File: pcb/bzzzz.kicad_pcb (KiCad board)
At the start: 2 copper layers, 18.3 x 46.2 mm, 29 parts, among them J1 OUT, J2 OUT, Q1 FDD8424H, Q2 FDD8424H

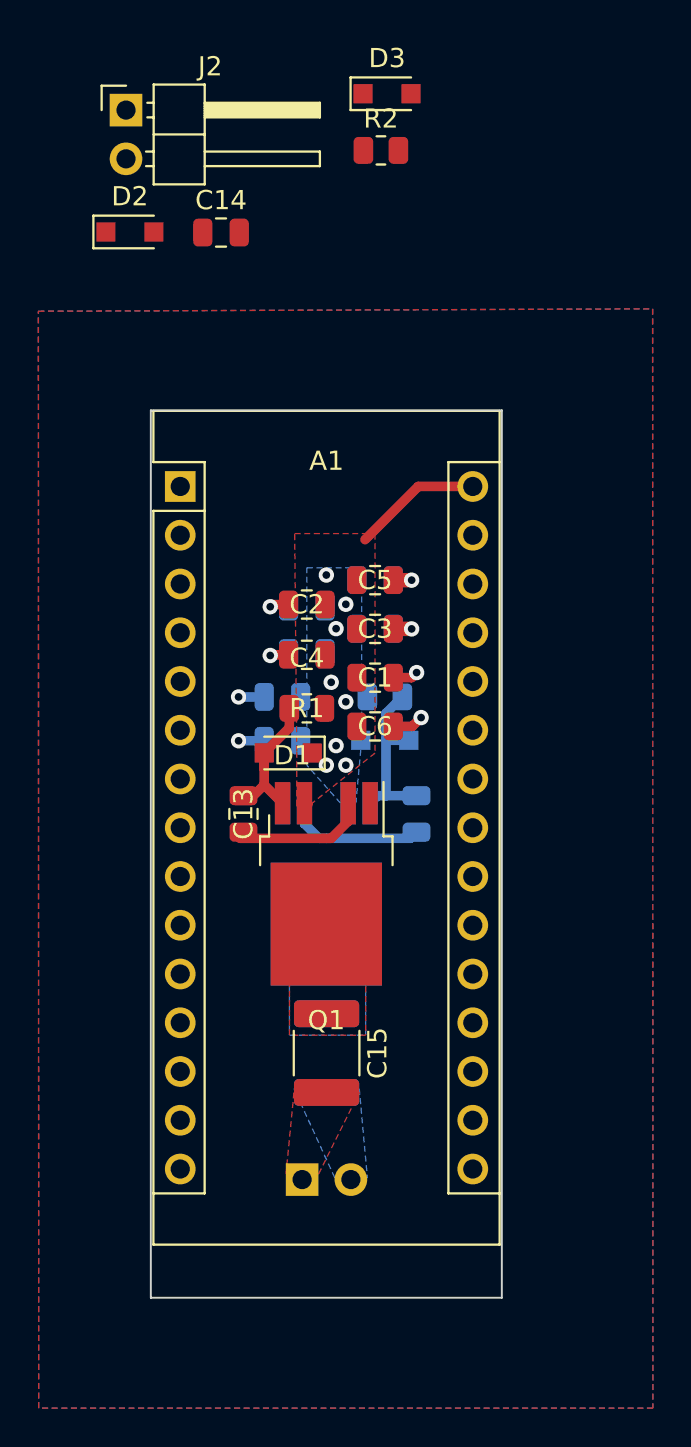
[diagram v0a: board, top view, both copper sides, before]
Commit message: pcb ordered from jlc
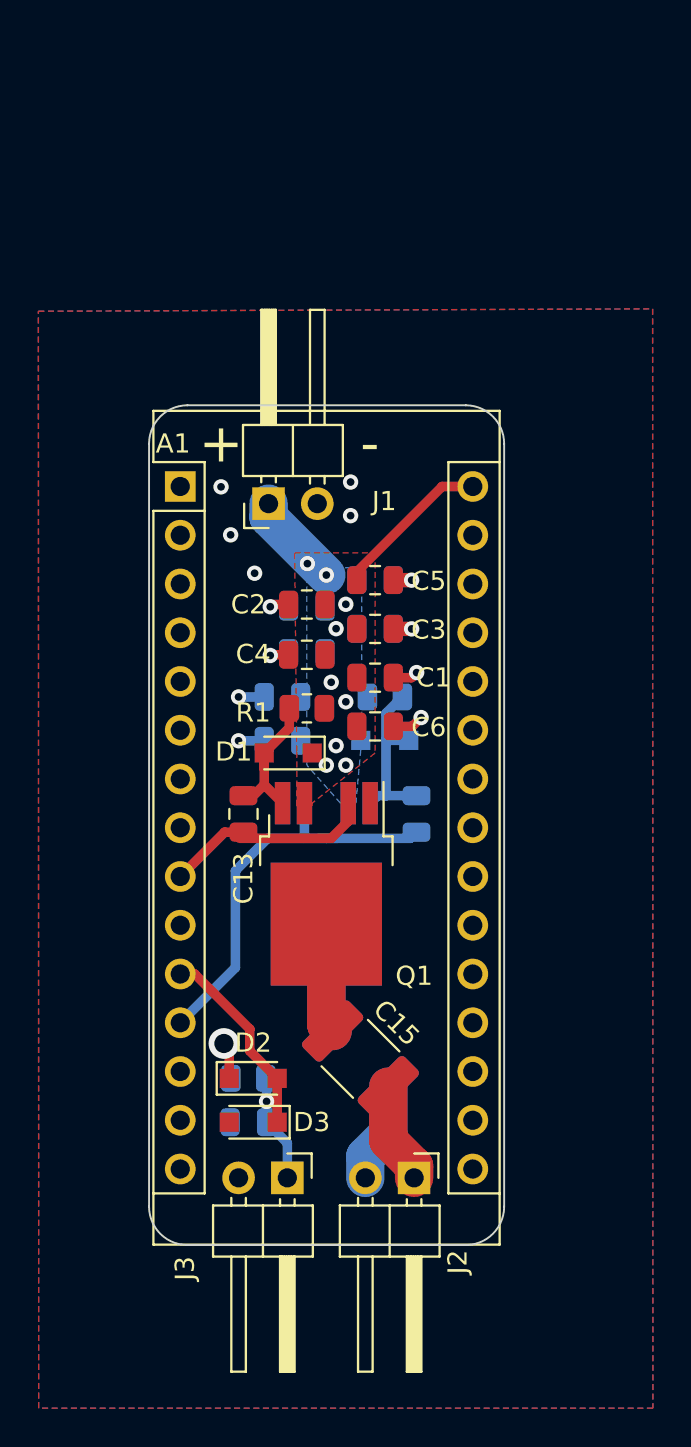
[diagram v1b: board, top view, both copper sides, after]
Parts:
- added J1: PWR, Connector_PinHeader_2.54mm:PinHeader_1x02_P2.54mm_Horizontal, F.Cu at (139.0, 117.1)
- C14, R2: moved to B.Cu
- J2: renamed from J1; moved to F.Cu
- J3: renamed from J2; value OUT -> ARC
- moved J3 56.3 mm to (140.0, 152.2), turned to -90 degrees
- moved D3 54.0 mm to (138.2, 149.4), turned to 180 degrees
- moved R2 48.8 mm to (137.9, 147.1), turned to 180 degrees
- moved C14 46.4 mm to (137.9, 149.4), turned to 180 degrees
- moved D2 44.6 mm to (138.2, 147.1)
- moved J2 5.83 mm to (146.6, 152.2)
- moved C15 1.79 mm to (143.8, 146.1), turned to -45 degrees
- moved C16 1.79 mm to (143.8, 146.1), turned to 135 degrees
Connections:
- A1 pad 11: unconnected-(A1-Pad11) -> /ARC_DETECT
- A1 pad 12: unconnected-(A1-Pad12) -> /PWM_B
- A1 pad 5: /ARC_DETECT -> unconnected-(A1-Pad5)
- A1 pad 6: /PWM_A -> unconnected-(A1-Pad6)
- A1 pad 7: /PWM_B -> unconnected-(A1-Pad7)
- A1 pad 9: unconnected-(A1-Pad9) -> /PWM_A
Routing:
- net /ARC_DETECT: track 0.00 -> 16.5 mm, vias 0 -> 1
- net /PWM_B: track 7.36 -> 23.2 mm
- net VCC: track 6.76 -> 13.3 mm, vias 8 -> 9
- net Net-(C16-Pad2): track 0.00 -> 5.71 mm
- net Net-(C15-Pad1): track 0.00 -> 5.71 mm
- net Net-(C15-Pad2): track 0.00 -> 5.31 mm
- net Net-(C16-Pad1): track 0.00 -> 5.25 mm
- net /PWM_A: track 6.96 -> 11.2 mm
- net +5V: track 0.00 -> 1.93 mm, vias 0 -> 1
- net GND: vias 8 -> 13
- removed copper zone on F.Cu, net Net-(C15-Pad1)
- removed copper zone on F.Cu, net Net-(C15-Pad2)
- removed copper zone on B.Cu, net Net-(C16-Pad1)
- removed copper zone on B.Cu, net Net-(C16-Pad2)
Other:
- board size 18.3 x 46.2 mm -> 18.5 x 43.8 mm
- board text added: "+"
- board text added: "-"
- board text added: "A"
- board text added: "AD"
- board text added: "B"
- board text added: "GND"
